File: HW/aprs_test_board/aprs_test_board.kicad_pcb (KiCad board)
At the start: 2 copper layers, 48.4 x 25.3 mm, 19 parts, among them J1 Conn_Coaxial, J2 Conn_01x06, J3 Conn_01x06, U1 Si4461, Y1 30M

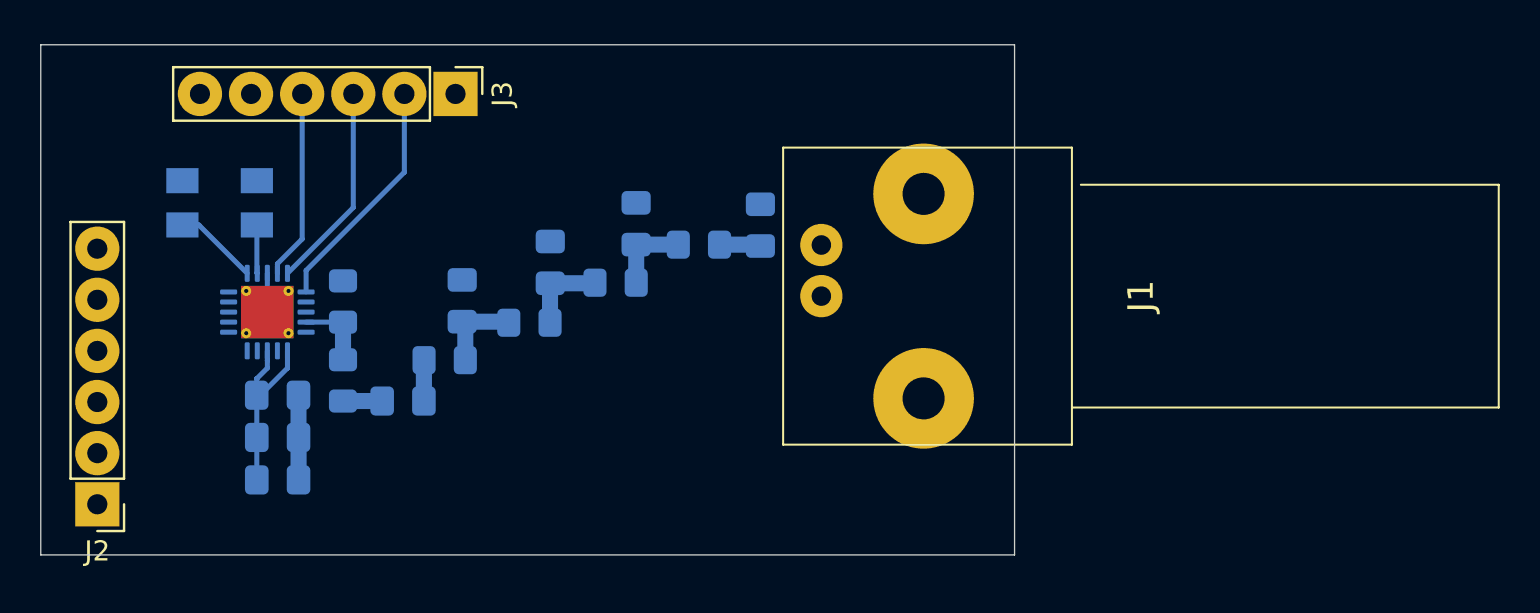
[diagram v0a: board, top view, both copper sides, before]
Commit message: APRS test board done
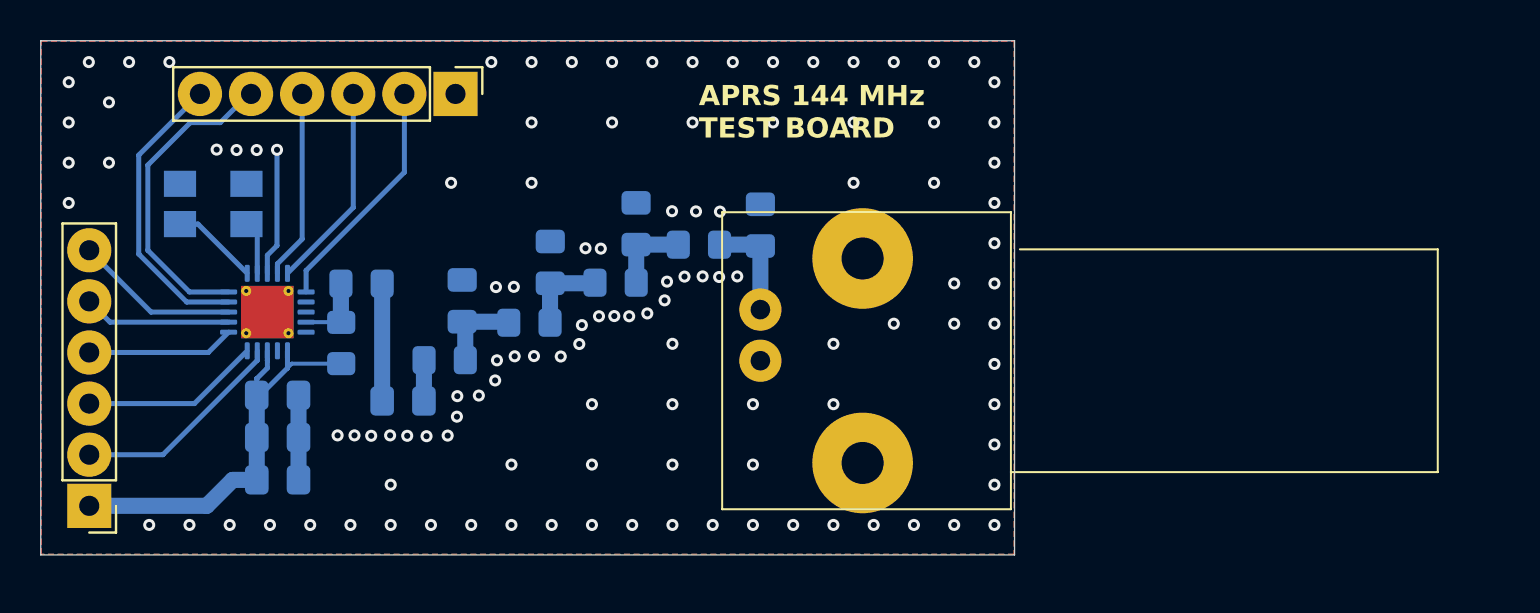
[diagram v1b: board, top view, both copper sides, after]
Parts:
- Y1: footprint Library:Crystal_SMD -> Crystal:Crystal_SMD_5032-4Pin_5.0x3.2mm
- moved L2 4.89 mm to (105.5, 102.0), turned to 0 degrees
- moved J1 4.41 mm to (125.4, 103.3)
- moved L1 2.06 mm to (104.5, 105.0), turned to 90 degrees
- moved J2 0.41 mm to (92.0, 113.0)
- moved Y1 0.33 mm to (98.2, 98.0)
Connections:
- J2 pad 1: GND -> +3.3V
- J3 pad 1: +3.3V -> GND
- U1 pad 10: Net-(J3-Pin_5) -> Net-(J2-Pin_3)
- U1 pad 11: Net-(J2-Pin_2) -> Net-(J2-Pin_4)
- U1 pad 12: Net-(J2-Pin_3) -> Net-(J2-Pin_5)
- U1 pad 13: Net-(J2-Pin_4) -> Net-(J2-Pin_6)
- U1 pad 14: Net-(J2-Pin_5) -> Net-(J3-Pin_6)
- U1 pad 15: Net-(J2-Pin_6) -> Net-(J3-Pin_5)
- U1 pad 9: Net-(J3-Pin_6) -> Net-(J2-Pin_2)
- Y1 pad 3: (no net) -> GND
- Y1 pad 4: (no net) -> GND
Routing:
- net Net-(J3-Pin_5): track 0.00 -> 15.7 mm
- net Net-(J3-Pin_6): track 0.00 -> 14.7 mm
- net +3.3V: track 9.59 -> 21.2 mm
- net Net-(J2-Pin_2): track 0.00 -> 10.8 mm
- net Net-(J2-Pin_3): track 0.00 -> 8.94 mm
- net Net-(J2-Pin_6): track 0.00 -> 8.20 mm
- net Net-(J2-Pin_5): track 0.00 -> 7.35 mm
- net Net-(J2-Pin_4): track 0.00 -> 7.34 mm
- net GND: track 6.20 -> 10.6 mm, vias 0 -> 117
- net Net-(C1-Pad1): track 1.95 -> 5.83 mm
- net Net-(J1-In): track 2.06 -> 5.22 mm
- added copper zone on B.Cu, net GND
- added copper zone on F.Cu, net GND
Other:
- board size 48.4 x 25.3 mm -> 48.4 x 25.5 mm
- board text added: "APRS 144 MHz TEST BOARD"

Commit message: test board
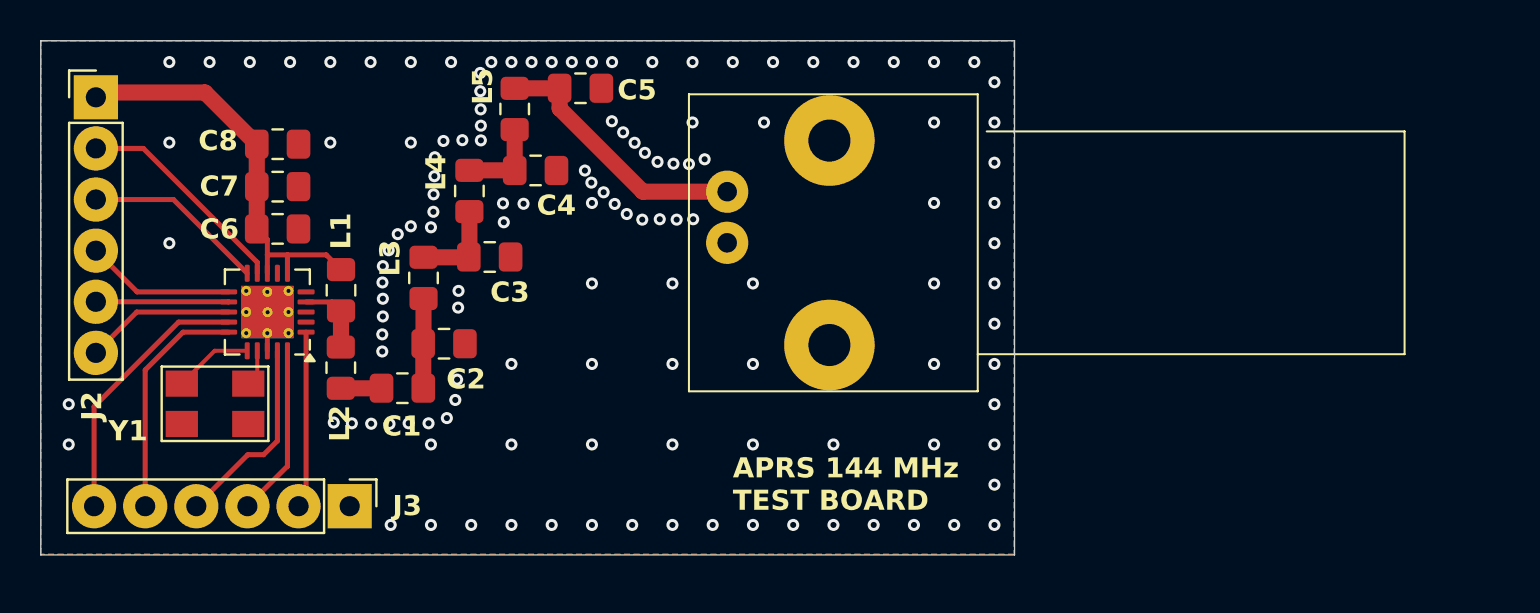
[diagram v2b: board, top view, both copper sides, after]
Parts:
- removed LX1: XX, Inductor_SMD:L_0805_2012Metric_Pad1.15x1.40mm_HandSolder
- added ?: , , F.Cu at (99.8, 103.4)
- added ?: , , F.Cu at (100.9, 104.5)
- added ?: , , F.Cu at (100.9, 103.4)
- added ?: , , F.Cu at (101.9, 103.4)
- added ?: , , F.Cu at (100.9, 102.4)
- C1, C2, C3, C4, C5, C6, C7, C8, L1, L2, L3, L4, L5, U1, Y1: moved to F.Cu
- moved J3 21.2 mm to (105.0, 113.1)
- moved J2 20.3 mm to (92.3, 92.8), turned to 0 degrees
- moved C8 16.7 mm to (101.4, 95.1)
- moved C7 12.5 mm to (101.4, 97.2)
- moved L5 11.4 mm to (113.2, 93.3), turned to 90 degrees
- moved C5 11.2 mm to (116.4, 92.3), turned to 180 degrees
- moved Y1 9.93 mm to (98.3, 108.0)
- moved L4 8.58 mm to (110.9, 97.4), turned to 90 degrees
- moved C6 8.26 mm to (101.4, 99.3)
- moved J1 6.09 mm to (123.7, 97.4)
- moved L3 5.71 mm to (108.6, 101.7), turned to 90 degrees
- moved C4 5.65 mm to (114.2, 96.4), turned to 180 degrees
- moved L2 4.30 mm to (104.5, 106.2), turned to -90 degrees
- moved C3 3.02 mm to (111.9, 100.7), turned to 180 degrees
- moved L1 2.62 mm to (104.5, 102.3), turned to -90 degrees
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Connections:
- C2 pad 2: Net-(C2-Pad2) -> Net-(C1-Pad2)
- L3 pad 1: Net-(C2-Pad2) -> Net-(C1-Pad2)
- Y1 pad 3: GND -> (no net)
- Y1 pad 4: GND -> (no net)
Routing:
- net GND: track 10.6 -> 0.88 mm, vias 117 -> 130
- net Net-(J1-In): track 5.22 -> 13.3 mm
- net Net-(C2-Pad2): track 4.31 -> 0.00 mm
- net Net-(J3-Pin_5): track 15.7 -> 11.7 mm
- net Net-(C1-Pad1): track 5.83 -> 2.02 mm
- net /SDN: track 11.9 -> 8.81 mm
- net Net-(C1-Pad2): track 2.03 -> 4.46 mm
- net Net-(J3-Pin_3): track 10.3 -> 8.55 mm
- net Net-(J3-Pin_6): track 14.7 -> 13.4 mm
- net Net-(U1-XIN): track 2.67 -> 1.82 mm
- net Net-(J2-Pin_6): track 8.20 -> 7.44 mm
- net Net-(J2-Pin_5): track 7.35 -> 6.60 mm
- net +3.3V: track 21.2 -> 20.6 mm
